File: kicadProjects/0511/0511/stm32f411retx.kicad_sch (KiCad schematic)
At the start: 16 parts, among them SW68 SW_Push, U8 STM32F411RETx, Y1 Crystal

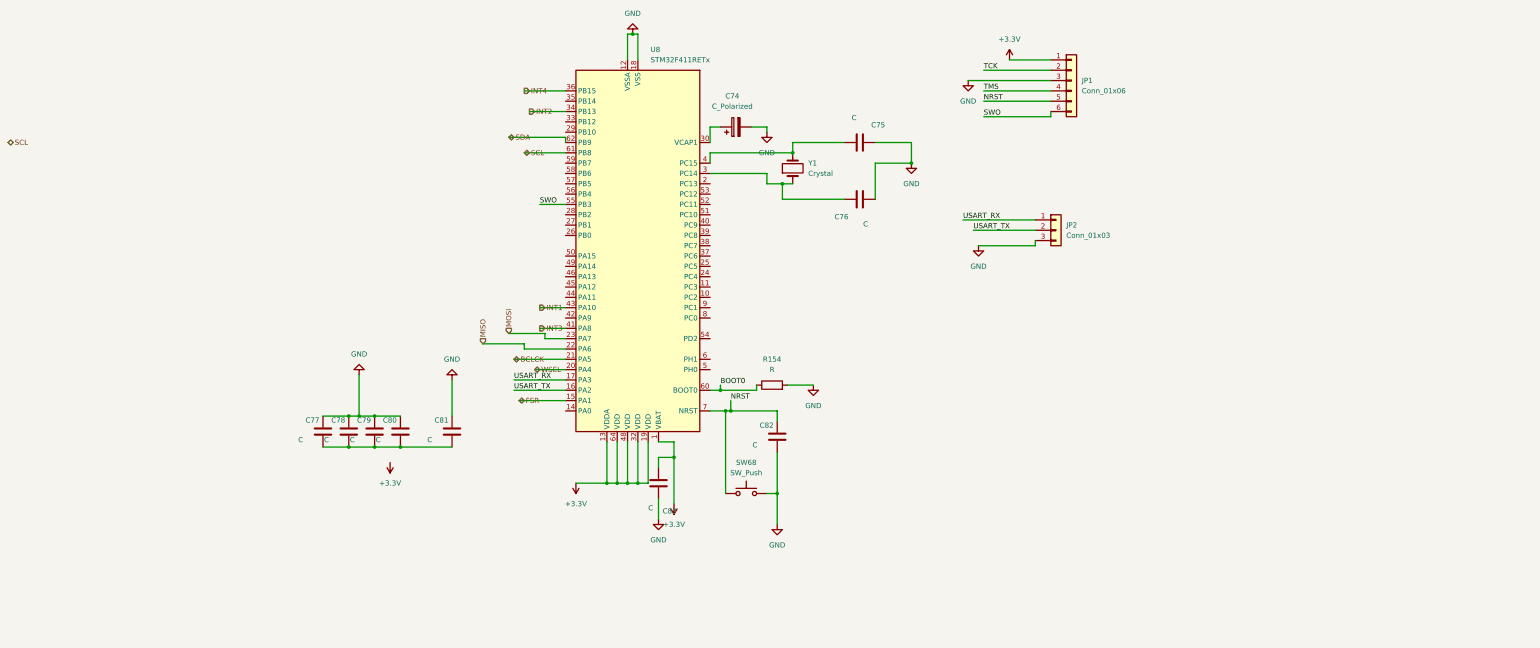
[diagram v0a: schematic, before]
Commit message: added comments
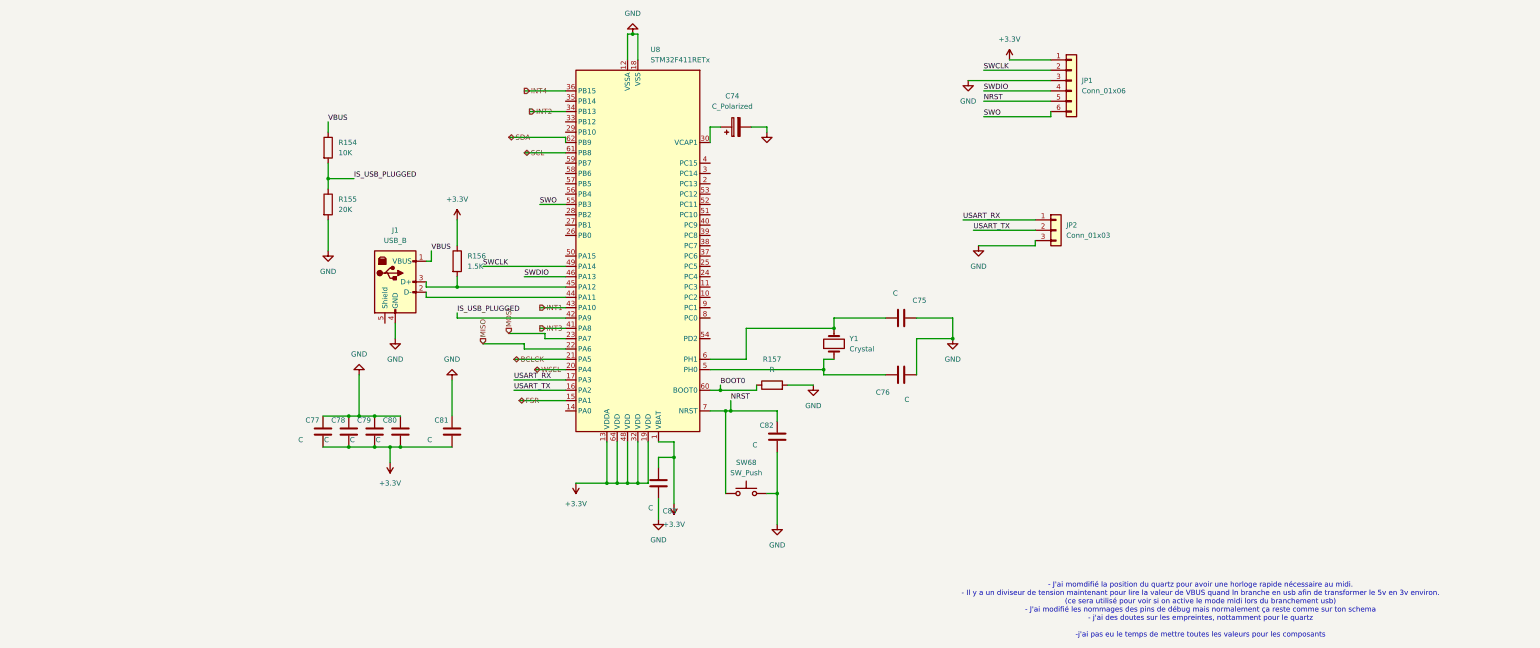
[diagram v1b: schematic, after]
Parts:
- added J1: USB_B, Connector_USB:USB_Micro-B_Molex_47346-0001, symbol Connector:USB_B
- added R154: 10K, Resistor_SMD:R_0603_1608Metric, symbol Device:R
- added R155: 20K, Resistor_SMD:R_0603_1608Metric, symbol Device:R
- added R156: 1.5K, Resistor_SMD:R_0603_1608Metric, symbol Device:R
- renumbered R154 to R157
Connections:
- net TCK is gone; now on net SWCLK: JP1.2 (Pin_2)
- net TMS is gone; now on net SWDIO: JP1.4 (Pin_4)
- net +3.3V: now also C77.2, C78.2, C79.2, C80.2, C81.2, R156.1
- net GND: now also J1.4 (GND), R155.2
- net at C75.2, Y1.2: now also U8.6 (PH1); no longer U8.4 (PC15)
- net at C76.1, Y1.1: now also U8.5 (PH0); no longer U8.3 (PC14)
- net IS_USB_PLUGGED: now reaches U8.42 (PA9)
- net IS_USB_PLUGGED: now also R154.2, R155.1
- net at U8.44 (PA11): now also J1.2 (D-)
- net at U8.45 (PA12): now also J1.3 (D+), R156.2
- net SWDIO: now reaches U8.46 (PA13)
- net SWCLK: now reaches U8.49 (PA14)
- new net VBUS: J1.1 (VBUS), R154.1
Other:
- note added: "- J'ai momdifié la position du quartz pour avoir une horloge rapide nécessaire au midi. - Il y a un diviseur de tension maintenant pour lire la valeur de VBUS quand ln branche en usb afin de transformer le 5v en 3v environ. (ce sera utilisé pour voir si on active le mode midi lors du branchement usb) - J'ai modifié les nommages des pins de débug mais normalement ça reste comme sur ton schema - j'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"
- moved on the sheet: C75, C76, Y1
